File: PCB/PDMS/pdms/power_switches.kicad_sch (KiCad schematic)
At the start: 8 parts

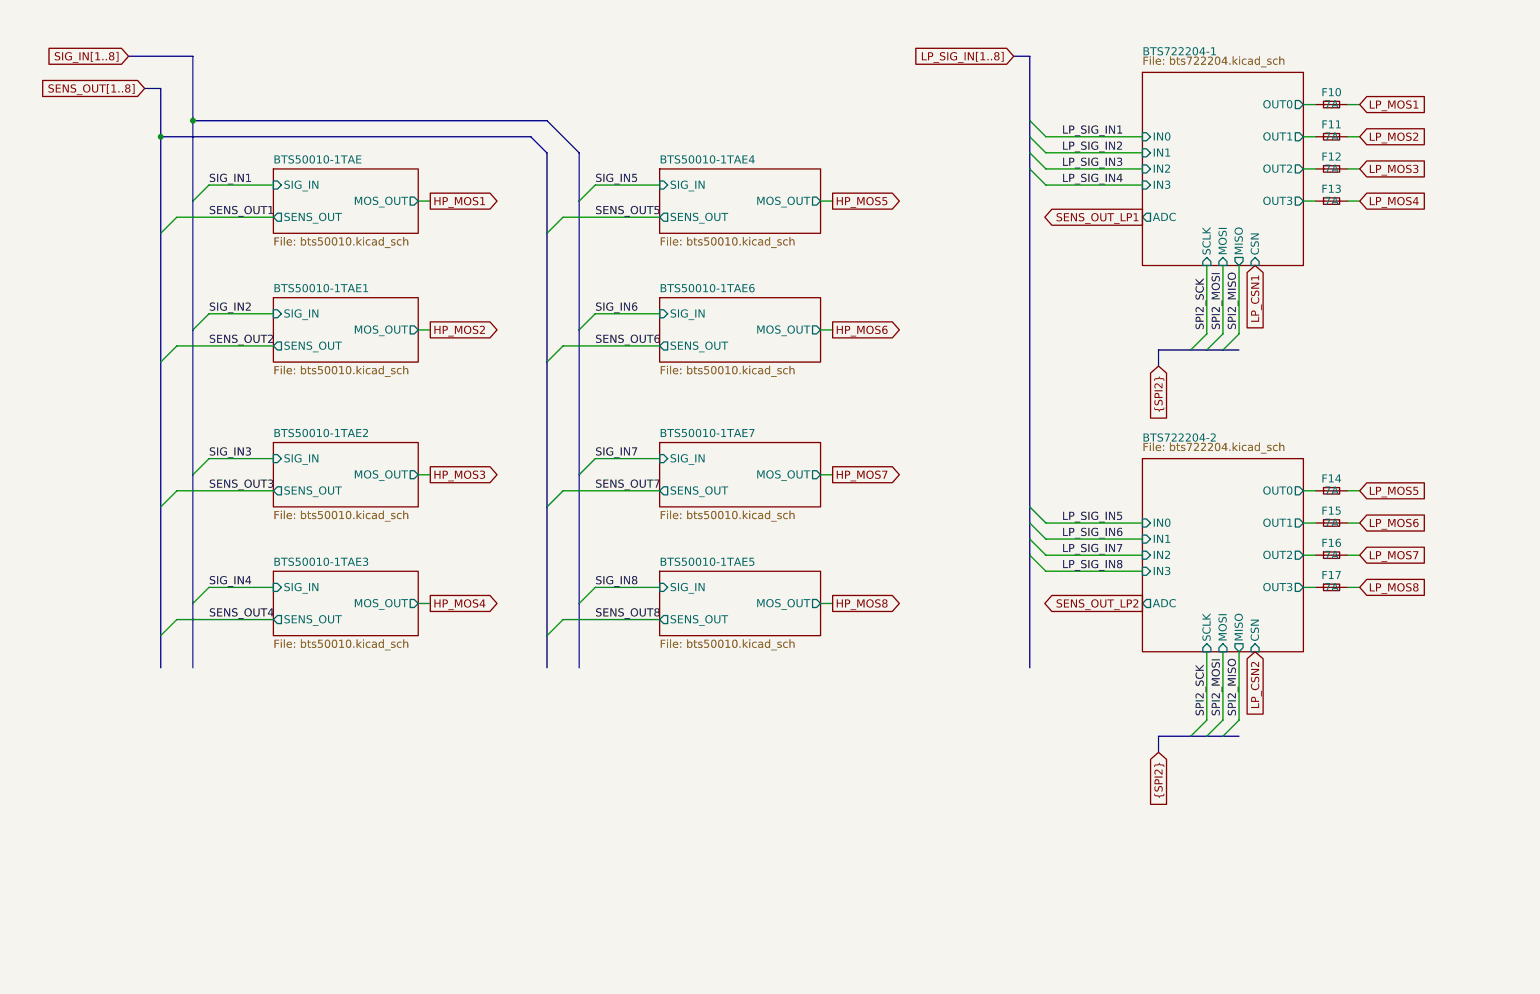
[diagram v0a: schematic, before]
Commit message: Major changes with new switch
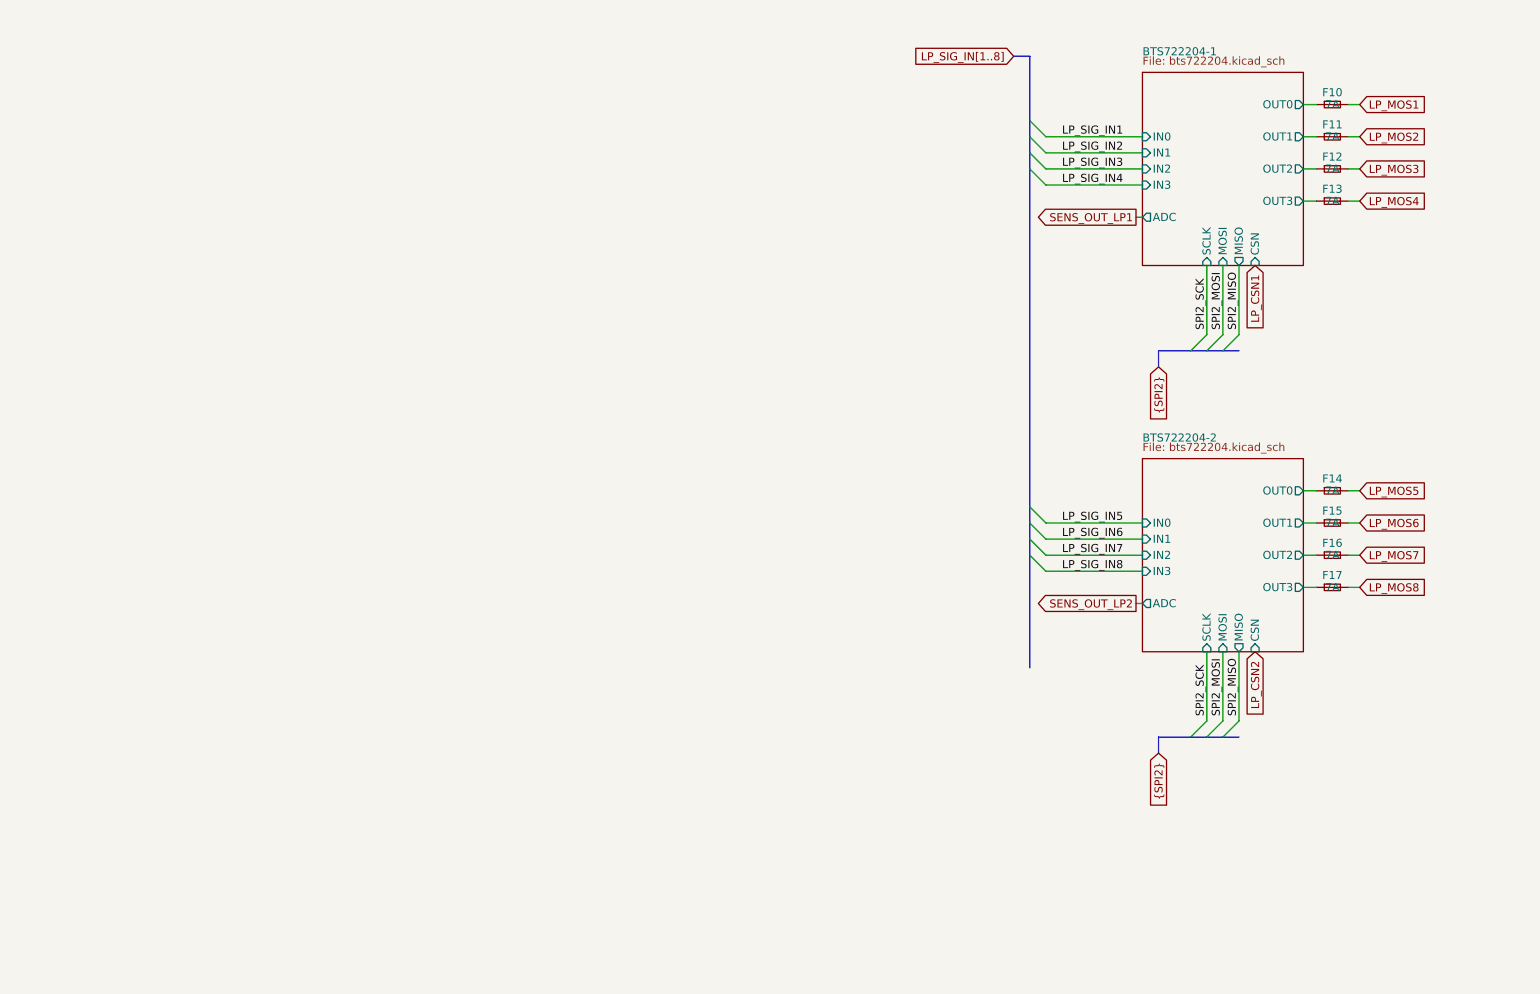
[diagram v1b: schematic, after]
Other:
- removed sheet BTS50010-1TAE
- removed sheet BTS50010-1TAE1
- removed sheet BTS50010-1TAE2
- removed sheet BTS50010-1TAE3
- removed sheet BTS50010-1TAE4
- removed sheet BTS50010-1TAE5
- removed sheet BTS50010-1TAE6
- removed sheet BTS50010-1TAE7

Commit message: Clean-up of schematics
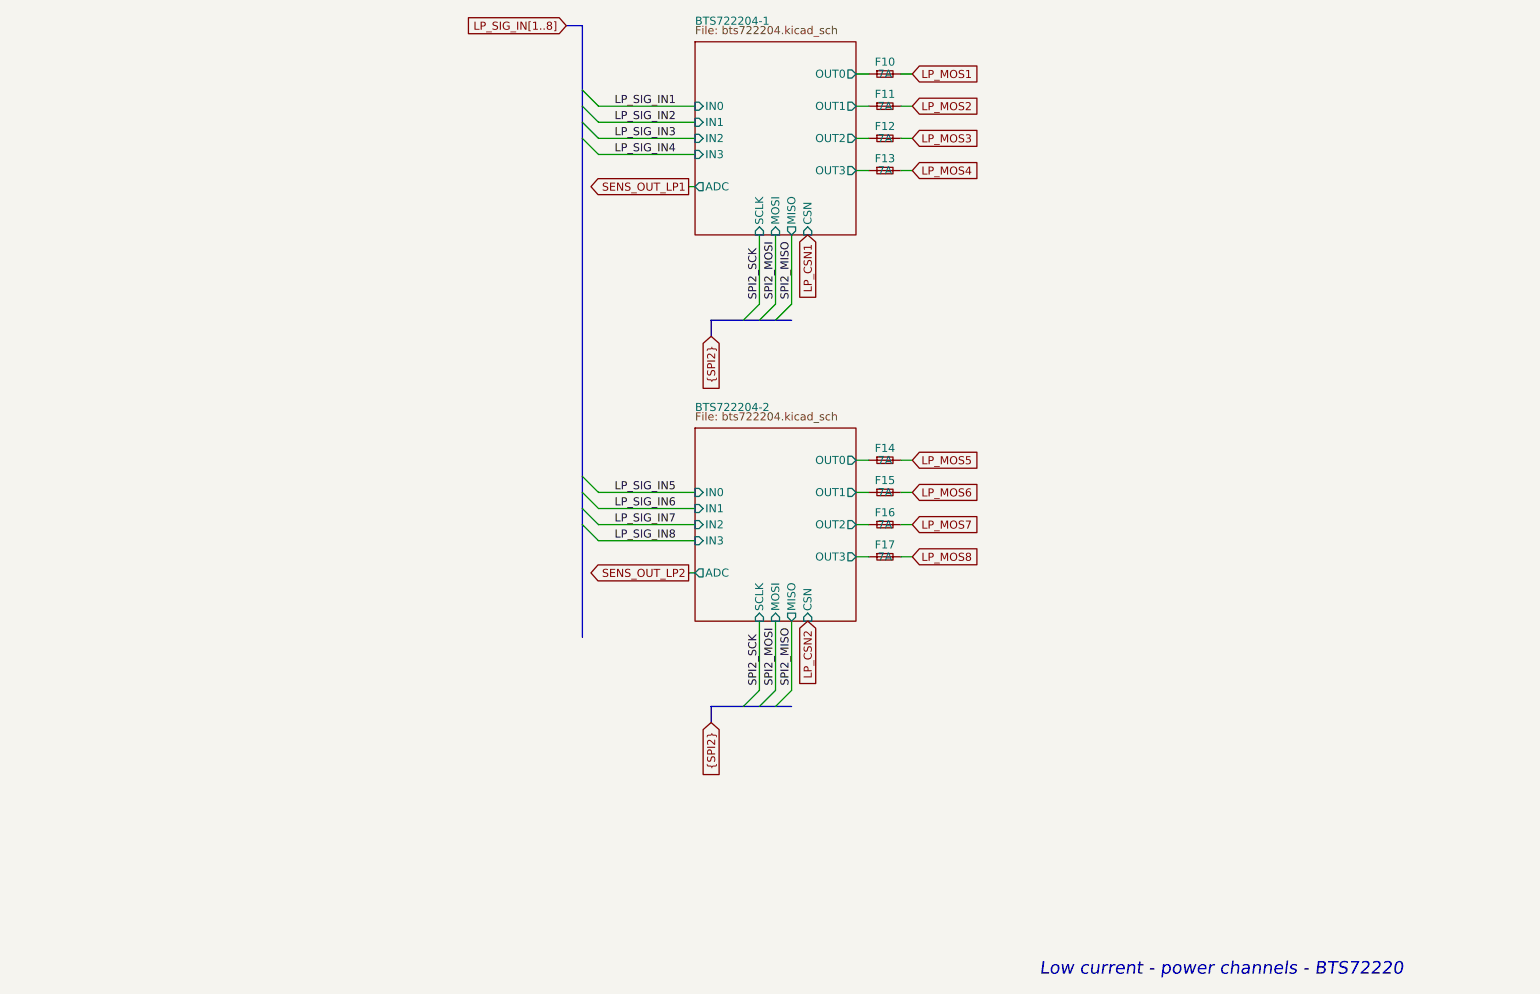
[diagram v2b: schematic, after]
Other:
- note added: "Low current - power channels - BTS72220"
- moved on the sheet: F10, F11, F12, F13, F14, F15, F16, F17
